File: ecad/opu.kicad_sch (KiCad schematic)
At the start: 5 parts, among them J1 Conn_01x24

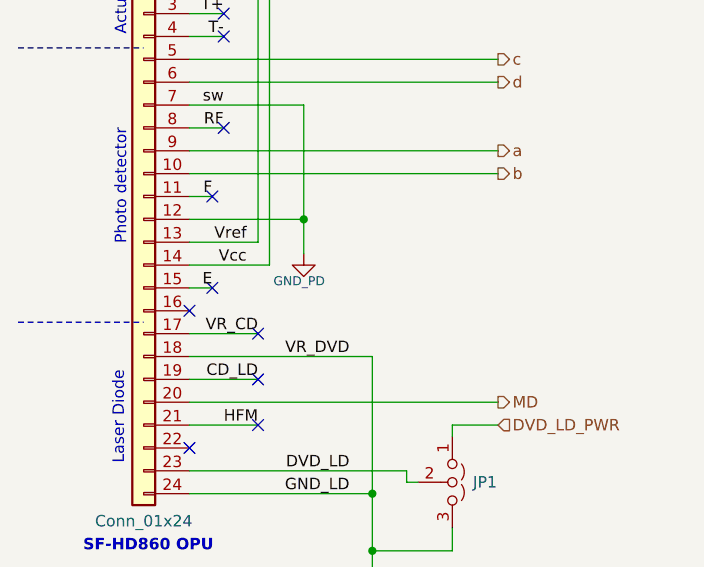
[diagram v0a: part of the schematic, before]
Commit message: need to sweep
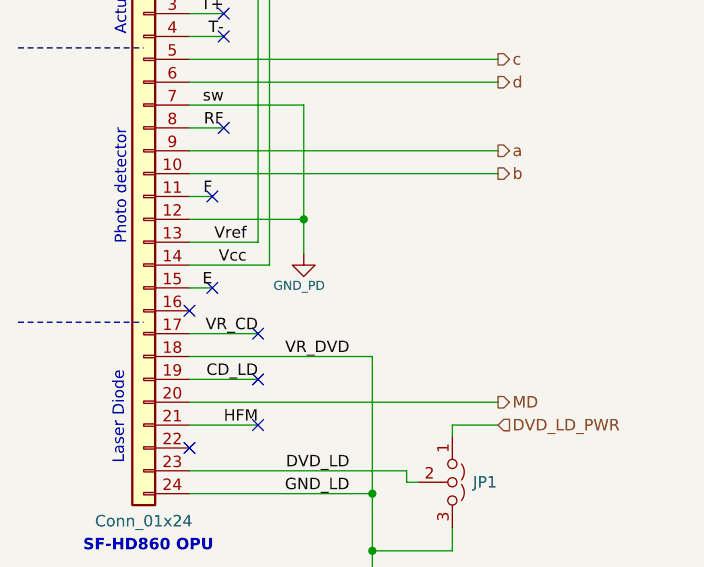
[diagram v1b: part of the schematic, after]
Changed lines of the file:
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@@
 		)
 		(property "Value" "GND_PD"
-			(at 141.732 105.918 0)
+			(at 141.732 106.426 0)
 			(show_name no)
 			(do_not_autoplace no)
